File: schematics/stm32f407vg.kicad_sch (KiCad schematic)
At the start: 15 parts, among them X2 8MHz

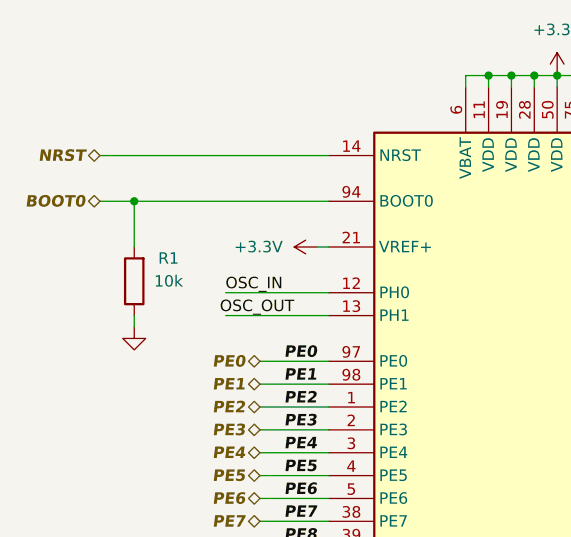
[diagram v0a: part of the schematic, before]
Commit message: Файлы измененный Kicad
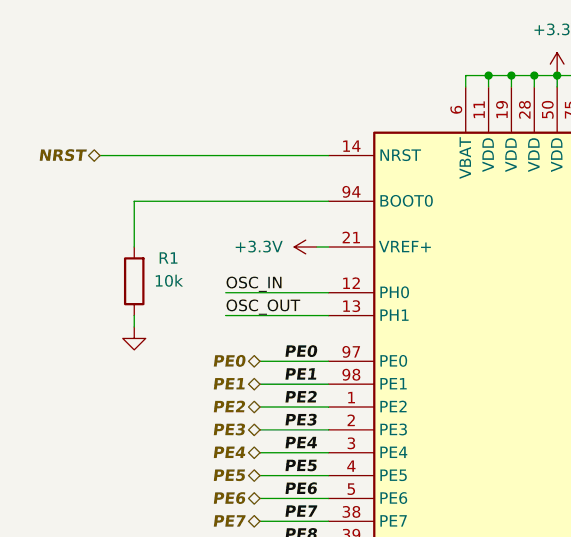
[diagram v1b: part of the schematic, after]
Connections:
- net BOOT0: no longer names the net of MK2.94 (BOOT0), R1.2
